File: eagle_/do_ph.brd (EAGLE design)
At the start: 100 x 80.6 mm, 26 parts, among them IC1 MEGA8-P, Q1 8Mhz

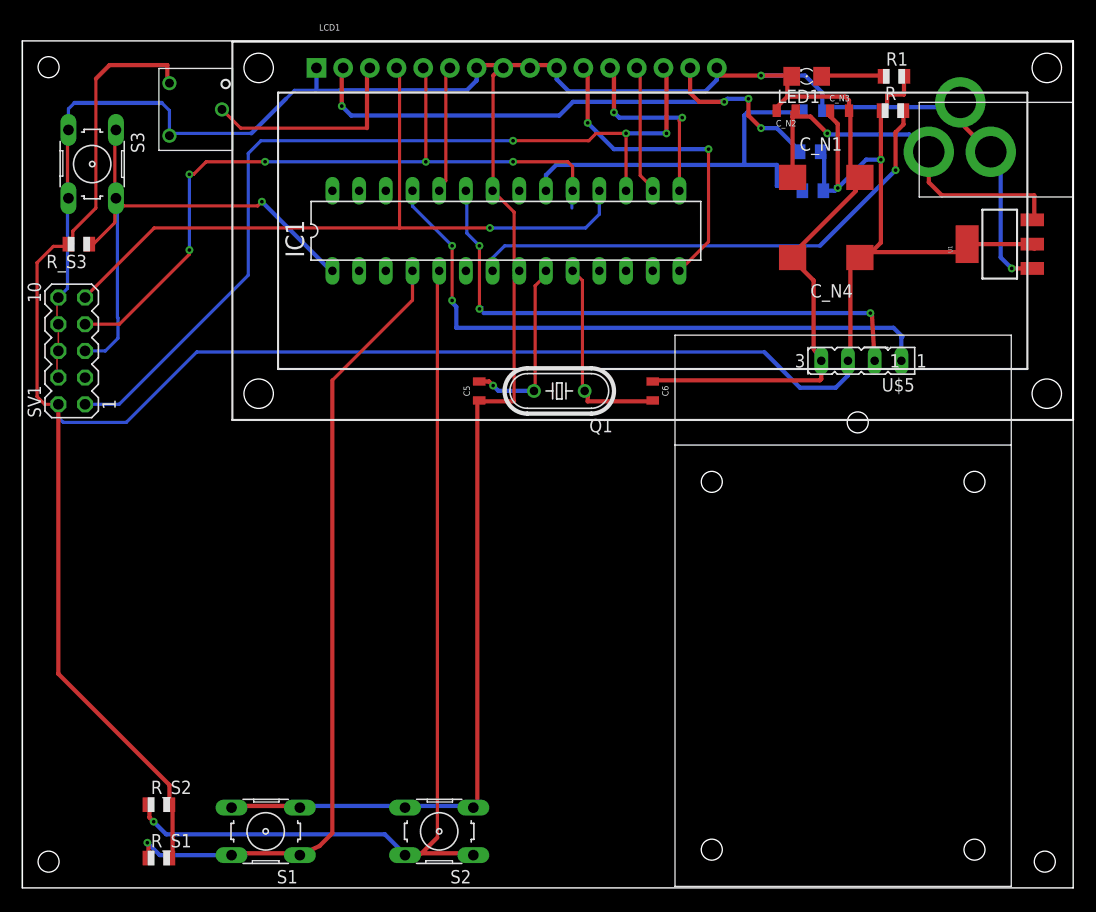
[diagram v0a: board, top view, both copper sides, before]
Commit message: update
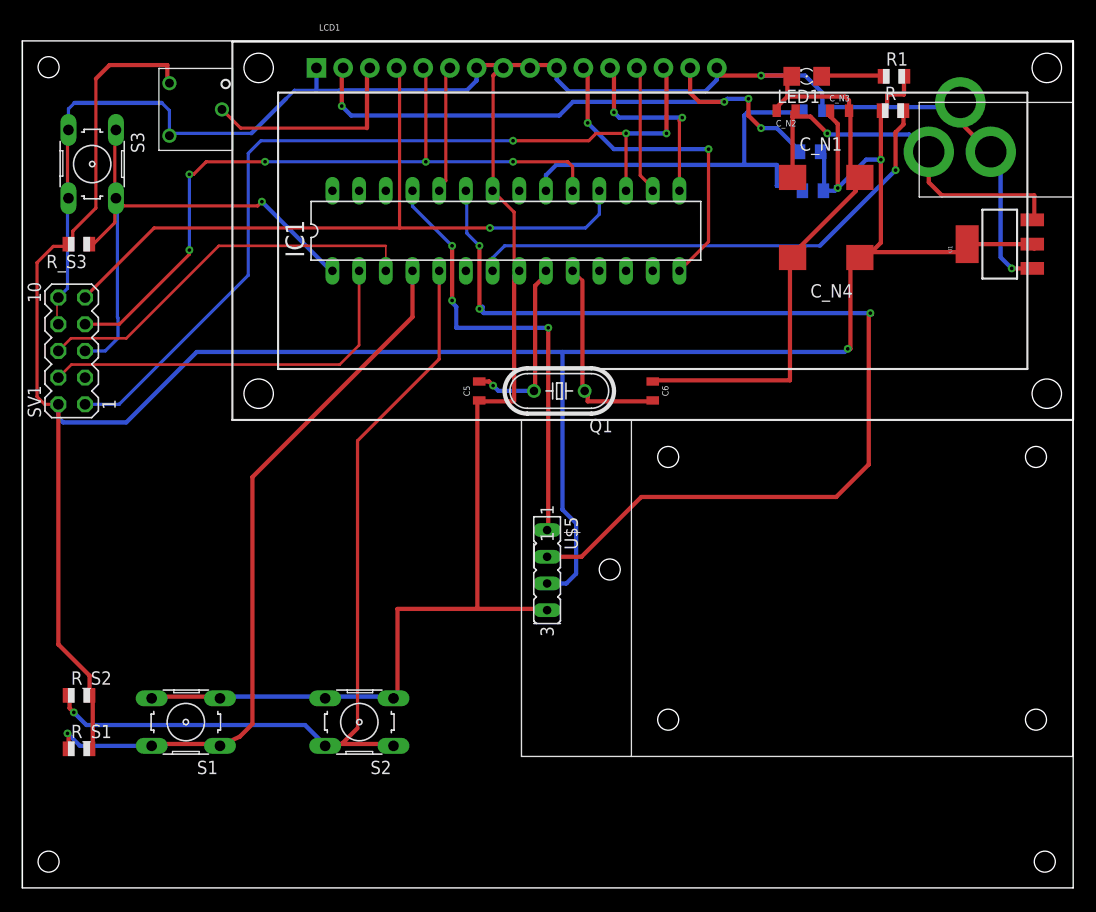
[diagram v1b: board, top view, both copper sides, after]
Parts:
- moved U$5 18.0 mm to (86.5, 29.4), turned to 180 degrees
- moved S1 12.9 mm to (15.3, 15.5)
- moved S2 12.9 mm to (31.8, 15.5)
- moved R_S1 12.9 mm to (5.10, 12.9)
- moved R_S2 12.9 mm to (5.10, 18.0)
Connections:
- new net RX: IC1.2, SV1.4
- new net TX: IC1.3, SV1.6
- net GND: no longer SV1.4, SV1.6
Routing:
- net ADC_1: track 54.2 -> 98.5 mm
- net TX: track 0.00 -> 37.9 mm
- net RX: track 0.00 -> 37.4 mm
- net ADC_2: track 60.0 -> 43.0 mm, vias 2 -> 3
- net START: track 77.1 -> 69.9 mm
- net START2: track 89.9 -> 82.6 mm
- net VCC: track 243.0 -> 250.2 mm, vias 2 -> 3
- net GND: track 308.5 -> 302.9 mm
- net RW: track 70.7 -> 69.1 mm

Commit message: update
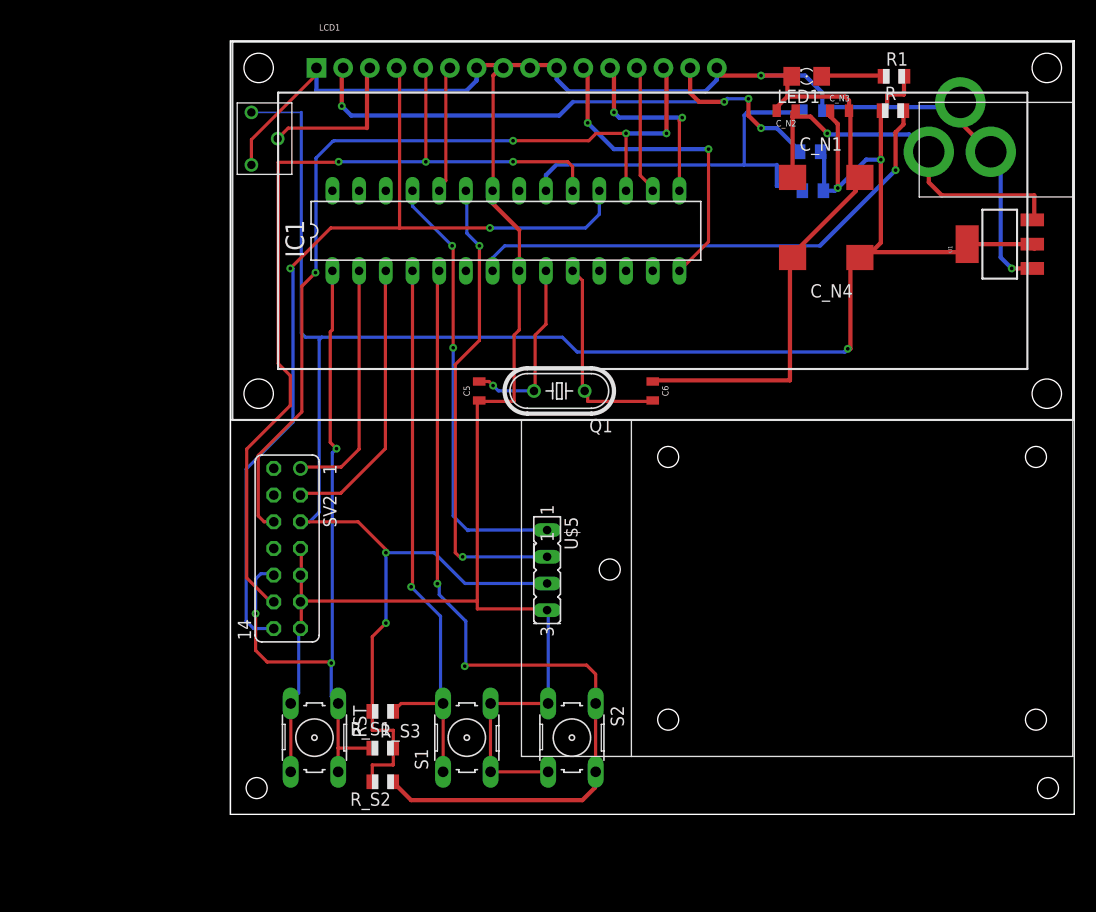
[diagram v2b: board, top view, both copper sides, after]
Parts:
- removed S3: (no value), switch-omron:B3F-10XX
- removed SV1: (no value), con-lstb:MA05-2
- removed U$6: RM065_V1, RM065:RM065
- added RST: (no value), switch-omron:B3F-10XX
- added SV2: (no value), con-lsta:FE07-2
- added U$2: RES_RM063, res_RM063:RM063
- moved R_S3 56.0 mm to (34.0, 13.0), turned to 0 degrees
- moved R_S2 30.0 mm to (34.0, 9.80), turned to 180 degrees
- moved R_S1 29.1 mm to (34.0, 16.5), turned to 180 degrees
- moved S1 26.8 mm to (42.0, 14.0), turned to 90 degrees
- moved S2 20.3 mm to (52.0, 14.0), turned to 270 degrees
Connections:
- net D7: now also SV2.6; no longer SV1.1
- net GND: now also RST.3, RST.4, SV2.11, SV2.13, SV2.7, SV2.9, U$2.P$2; no longer S3.3, S3.4, SV1.10, SV1.8, U$6.P$2
- net N$1: now also U$2.P$3; no longer U$6.P$3
- net RS: now also SV2.14; no longer SV1.9
- net RST: now also RST.1, RST.2, SV2.10; no longer S3.1, S3.2, SV1.5
- net RW: now also SV2.12; no longer SV1.7
- net RX: now also SV2.1; no longer SV1.4
- net TX: now also SV2.3; no longer SV1.6
- net VCC: now also SV2.5, U$2.P$1; no longer SV1.2, U$6.P$1
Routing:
- net ADC_1: track 98.5 -> 44.9 mm, vias 3 -> 2
- net VCC: track 250.2 -> 215.2 mm, vias 3 -> 5
- net RS: track 69.8 -> 87.7 mm, vias 1 -> 2
- net RST: track 52.9 -> 68.9 mm, vias 1 -> 3
- net START: track 69.9 -> 54.1 mm
- net RW: track 69.1 -> 84.9 mm, vias 5 -> 3
- net RX: track 37.4 -> 23.5 mm
- net GND: track 302.9 -> 290.6 mm
- net TX: track 37.9 -> 26.9 mm
- net N$1: track 20.4 -> 14.8 mm
- net ADC_2: track 43.0 -> 42.2 mm, vias 3 -> 2
- net D7: track 84.9 -> 84.2 mm, vias 3 -> 4
- net START2: track 82.6 -> 83.2 mm, vias 1 -> 2
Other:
- board size 100 x 80.6 mm -> 80.3 x 73.6 mm
